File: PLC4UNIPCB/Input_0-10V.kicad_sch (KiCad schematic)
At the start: 3 parts

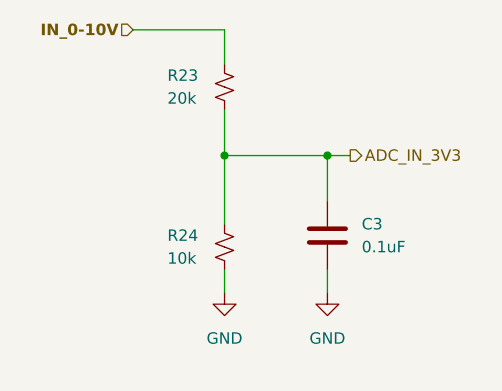
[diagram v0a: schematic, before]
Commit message: Add files via upload
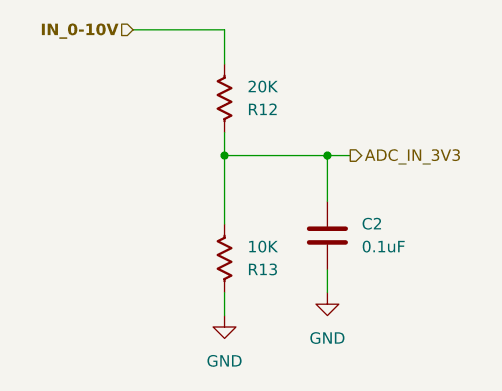
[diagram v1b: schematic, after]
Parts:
- removed R23: 20k, PCM_SparkFun-Resistor:R_0603_1608Metric, symbol PCM_SparkFun-Resistor:4.7k_0603
- removed R24: 10k, PCM_SparkFun-Resistor:R_0603_1608Metric, symbol PCM_SparkFun-Resistor:4.7k_0603
- added R12: 20K, PCM_Resistor_SMD_AKL:R_0603_1608Metric, symbol GP8211S-TC50:R_0603
- added R13: 10K, PCM_Resistor_SMD_AKL:R_0603_1608Metric, symbol GP8211S-TC50:R_0603
- renumbered C3 to C2
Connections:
- net ADC_IN_3V3: now also R12.2, R13.1
- net GND: now also R13.2
- net IN_0-10V: now also R12.1
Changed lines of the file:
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@@
 	(paper "A4")
+	(junction
+		(at 96.52 57.15)
+		(diameter 0)
+		(color 0 0 0 0)
+	)
 	(junction
 		(at 107.95 57.15)
@@
 		(color 0 0 0 0)
 	)
-	(junction
-		(at 96.52 57.15)
-		(diameter 0)
-		(color 0 0 0 0)
-	)
-	(wire
-		(pts
-			(xy 96.52 69.85) (xy 96.52 72.39)
+	(wire
+		(pts
+			(xy 96.52 72.39) (xy 96.52 74.93)
 		)
 		(stroke
@@
 	(wire
 		(pts
-			(xy 96.52 52.07) (xy 96.52 57.15)
-		)
-		(stroke
-			(width 0)
-			(type default)
-		)
-	)
-	(wire
-		(pts
 			(xy 96.52 57.15) (xy 107.95 57.15)
 		)
@@
 		(pts
 			(xy 96.52 43.18) (xy 96.52 46.99)
+		)
+		(stroke
+			(width 0)
+			(type default)
+		)
+	)
+	(wire
+		(pts
+			(xy 96.52 54.61) (xy 96.52 57.15)
 		)
 		(stroke
@@
 		(dnp no)
 		(fields_autoplaced yes)
-		(property "Reference" "#PWR035"
+		(property "Reference" "#PWR021"
 			(at 107.95 78.74 0)
 			(effects
@@
 			(project "PLC4UNIPCB"
 				(path "/20dd9fa8-33e5-4e01-8b4a-8cb5828152c9/ef44eee8-cd41-4527-92e2-6c408c0d0d91/82682a40-f2c8-4ae2-a13e-2b4ac848d816"
-					(reference "#PWR035")
+					(reference "#PWR021")
 					(unit 1)
 				)
@@
 	)
 	(symbol
-		(lib_id "PCM_SparkFun-Resistor:4.7k_0603")
-		(at 96.52 49.53 90)
+		(lib_id "GP8211S-TC50:R_0603")
+		(at 96.52 50.8 0)
+		(mirror y)
 		(unit 1)
 		(exclude_from_sim no)
@@
 		(on_board yes)
 		(dnp no)
-		(property "Reference" "R23"
-			(at 90.17 48.26 90)
-			(effects
-				(font
-					(size 1.27 1.27)
-				)
-				(justify right)
-			)
-		)
-		(property "Value" "20k"
-			(at 90.17 50.8 90)
-			(effects
-				(font
-					(size 1.27 1.27)
-				)
-				(justify right)
-			)
-		)
-		(property "Footprint" "PCM_SparkFun-Resistor:R_0603_1608Metric"
-			(at 100.838 49.53 0)
-			(effects
-				(font
-					(size 1.27 1.27)
-				)
-				(hide yes)
-			)
-		)
-		(property "Datasheet" "https://www.vishay.com/docs/20035/dcrcwe3.pdf"
-			(at 105.41 49.53 0)
-			(effects
-				(font
-					(size 1.27 1.27)
-				)
-				(hide yes)
-			)
-		)
-		(property "Description" "Resistor"
-			(at 107.95 49.53 0)
-			(effects
-				(font
-					(size 1.27 1.27)
-				)
-				(hide yes)
-			)
-		)
-		(property "PROD_ID" "RES-07857"
-			(at 103.124 49.53 0)
-			(effects
-				(font
-					(size 1.27 1.27)
-				)
-				(hide yes)
-			)
-		)
-		(property "LCSC" "C99782"
-			(at 96.52 49.53 90)
-			(effects
-				(font
-					(size 1.27 1.27)
-				)
-				(hide yes)
-			)
+		(property "Reference" "R12"
+			(at 99.06 52.0701 0)
+			(effects
+				(font
+					(size 1.27 1.27)
+				)
+				(justify right)
+			)
+		)
+		(property "Value" "20K"
+			(at 99.06 49.5301 0)
+			(effects
+				(font
+					(size 1.27 1.27)
+				)
+				(justify right)
+			)
+		)
+		(property "Footprint" "PCM_Resistor_SMD_AKL:R_0603_1608Metric"
+			(at 96.52 62.23 0)
+			(effects
+				(font
+					(size 1.27 1.27)
+				)
+				(hide yes)
+			)
+		)
+		(property "Datasheet" "~"
+			(at 96.52 50.8 0)
+			(effects
+				(font
+					(size 1.27 1.27)
+				)
+				(hide yes)
+			)
+		)
+		(property "Description" "SMD 0603 Chip Resistor, US Symbol, Alternate KiCad Library"
+			(at 96.52 50.8 0)
+			(effects
+				(font
+					(size 1.27 1.27)
+				)
+				(hide yes)
+			)
+		)
+		(property "LCSC" ""
+			(at 96.52 50.8 0)
+			(effects
+				(font
+					(size 1.27 1.27)
+				)
+				(hide yes)
+			)
+		)
+		(pin "1"
 		)
 		(pin "2"
-		)
-		(pin "1"
 		)
 		(instances
 			(project "PLC4UNIPCB"
 				(path "/20dd9fa8-33e5-4e01-8b4a-8cb5828152c9/ef44eee8-cd41-4527-92e2-6c408c0d0d91/82682a40-f2c8-4ae2-a13e-2b4ac848d816"
-					(reference "R23")
+					(reference "R12")
 					(unit 1)
 				)
@@
 	)
 	(symbol
-		(lib_id "PCM_SparkFun-Resistor:4.7k_0603")
-		(at 96.52 67.31 90)
+		(lib_id "GP8211S-TC50:R_0603")
+		(at 96.52 68.58 0)
+		(mirror y)
 		(unit 1)
 		(exclude_from_sim no)
@@
 		(on_board yes)
 		(dnp no)
-		(property "Reference" "R24"
-			(at 90.17 66.04 90)
-			(effects
-				(font
-					(size 1.27 1.27)
-				)
-				(justify right)
-			)
-		)
-		(property "Value" "10k"
-			(at 90.17 68.58 90)
-			(effects
-				(font
-					(size 1.27 1.27)
-				)
-				(justify right)
-			)
-		)
-		(property "Footprint" "PCM_SparkFun-Resistor:R_0603_1608Metric"
-			(at 100.838 67.31 0)
-			(effects
-				(font
-					(size 1.27 1.27)
-				)
-				(hide yes)
-			)
-		)
-		(property "Datasheet" "https://www.vishay.com/docs/20035/dcrcwe3.pdf"
-			(at 105.41 67.31 0)
-			(effects
-				(font
-					(size 1.27 1.27)
-				)
-				(hide yes)
-			)
-		)
-		(property "Description" "Resistor"
-			(at 107.95 67.31 0)
-			(effects
-				(font
-					(size 1.27 1.27)
-				)
-				(hide yes)
-			)
-		)
-		(property "PROD_ID" "RES-07857"
-			(at 103.124 67.31 0)
-			(effects
-				(font
-					(size 1.27 1.27)
-				)
-				(hide yes)
-			)
-		)
-		(property "LCSC" "C99782"
-			(at 96.52 67.31 90)
-			(effects
-				(font
-					(size 1.27 1.27)
-				)
-				(hide yes)
-			)
+		(property "Reference" "R13"
+			(at 99.06 69.8501 0)
+			(effects
+				(font
+					(size 1.27 1.27)
+				)
+				(justify right)
+			)
+		)
+		(property "Value" "10K"
+			(at 99.06 67.3101 0)
+			(effects
+				(font
+					(size 1.27 1.27)
+				)
+				(justify right)
+			)
+		)
+		(property "Footprint" "PCM_Resistor_SMD_AKL:R_0603_1608Metric"
+			(at 96.52 80.01 0)
+			(effects
+				(font
+					(size 1.27 1.27)
+				)
+				(hide yes)
+			)
+		)
+		(property "Datasheet" "~"
+			(at 96.52 68.58 0)
+			(effects
+				(font
+					(size 1.27 1.27)
+				)
+				(hide yes)
+			)
+		)
+		(property "Description" "SMD 0603 Chip Resistor, US Symbol, Alternate KiCad Library"
+			(at 96.52 68.58 0)
+			(effects
+				(font
+					(size 1.27 1.27)
+				)
+				(hide yes)
+			)
+		)
+		(property "LCSC" ""
+			(at 96.52 68.58 0)
+			(effects
+				(font
+					(size 1.27 1.27)
+				)
+				(hide yes)
+			)
+		)
+		(pin "1"
 		)
 		(pin "2"
-		)
-		(pin "1"
 		)
 		(instances
 			(project "PLC4UNIPCB"
 				(path "/20dd9fa8-33e5-4e01-8b4a-8cb5828152c9/ef44eee8-cd41-4527-92e2-6c408c0d0d91/82682a40-f2c8-4ae2-a13e-2b4ac848d816"
-					(reference "R24")
+					(reference "R13")
 					(unit 1)
 				)
@@
 		(dnp no)
 		(fields_autoplaced yes)
-		(property "Reference" "C3"
+		(property "Reference" "C2"
 			(at 111.76 64.7699 0)
 			(effects
@@
 			(project "PLC4UNIPCB"
 				(path "/20dd9fa8-33e5-4e01-8b4a-8cb5828152c9/ef44eee8-cd41-4527-92e2-6c408c0d0d91/82682a40-f2c8-4ae2-a13e-2b4ac848d816"
-					(reference "C3")
+					(reference "C2")
 					(unit 1)
 				)
@@
 	(symbol
 		(lib_id "power:GND")
-		(at 96.52 72.39 0)
+		(at 96.52 74.93 0)
 		(unit 1)
 		(exclude_from_sim no)
@@
 		(dnp no)
 		(fields_autoplaced yes)
-		(property "Reference" "#PWR034"
-			(at 96.52 78.74 0)
+		(property "Reference" "#PWR020"
+			(at 96.52 81.28 0)
 			(effects
 				(font
@@
 		)
 		(property "Value" "GND"
-			(at 96.52 77.47 0)
+			(at 96.52 80.01 0)
 			(effects
 				(font
@@
 		)
 		(property "Footprint" ""
-			(at 96.52 72.39 0)
+			(at 96.52 74.93 0)
 			(effects
 				(font
@@
 		)
 		(property "Datasheet" ""
-			(at 96.52 72.39 0)
+			(at 96.52 74.93 0)
 			(effects
 				(font
@@
 		)
 		(property "Description" "Power symbol creates a global label with name \"GND\" , ground"
-			(at 96.52 72.39 0)
+			(at 96.52 74.93 0)
 			(effects
 				(font
@@
 			(project ""
 				(path "/20dd9fa8-33e5-4e01-8b4a-8cb5828152c9/ef44eee8-cd41-4527-92e2-6c408c0d0d91/82682a40-f2c8-4ae2-a13e-2b4ac848d816"
-					(reference "#PWR034")
+					(reference "#PWR020")
 					(unit 1)
 				)
